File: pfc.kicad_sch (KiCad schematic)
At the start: 58 parts, among them Q3 IRF740, U1 LM324, U2 LMV7219M5, U3 TC4427, U5 74HC00, U6 74LVC1G08

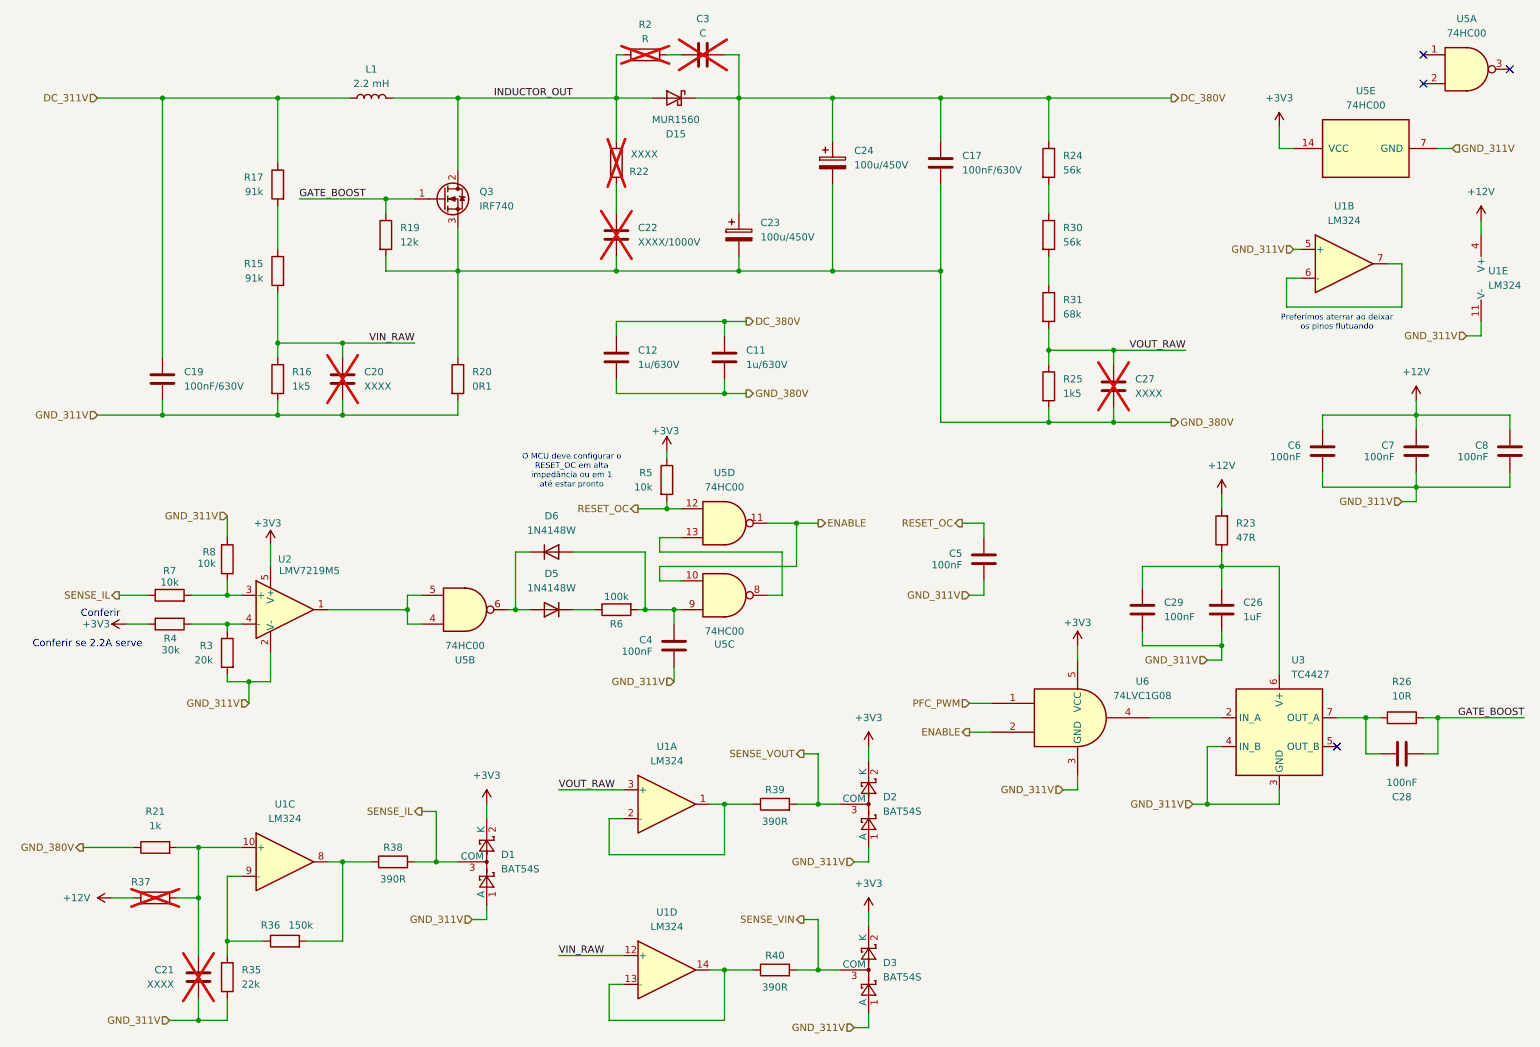
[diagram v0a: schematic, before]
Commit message: pcb: atualizar layout 2D da placa e esquematicos
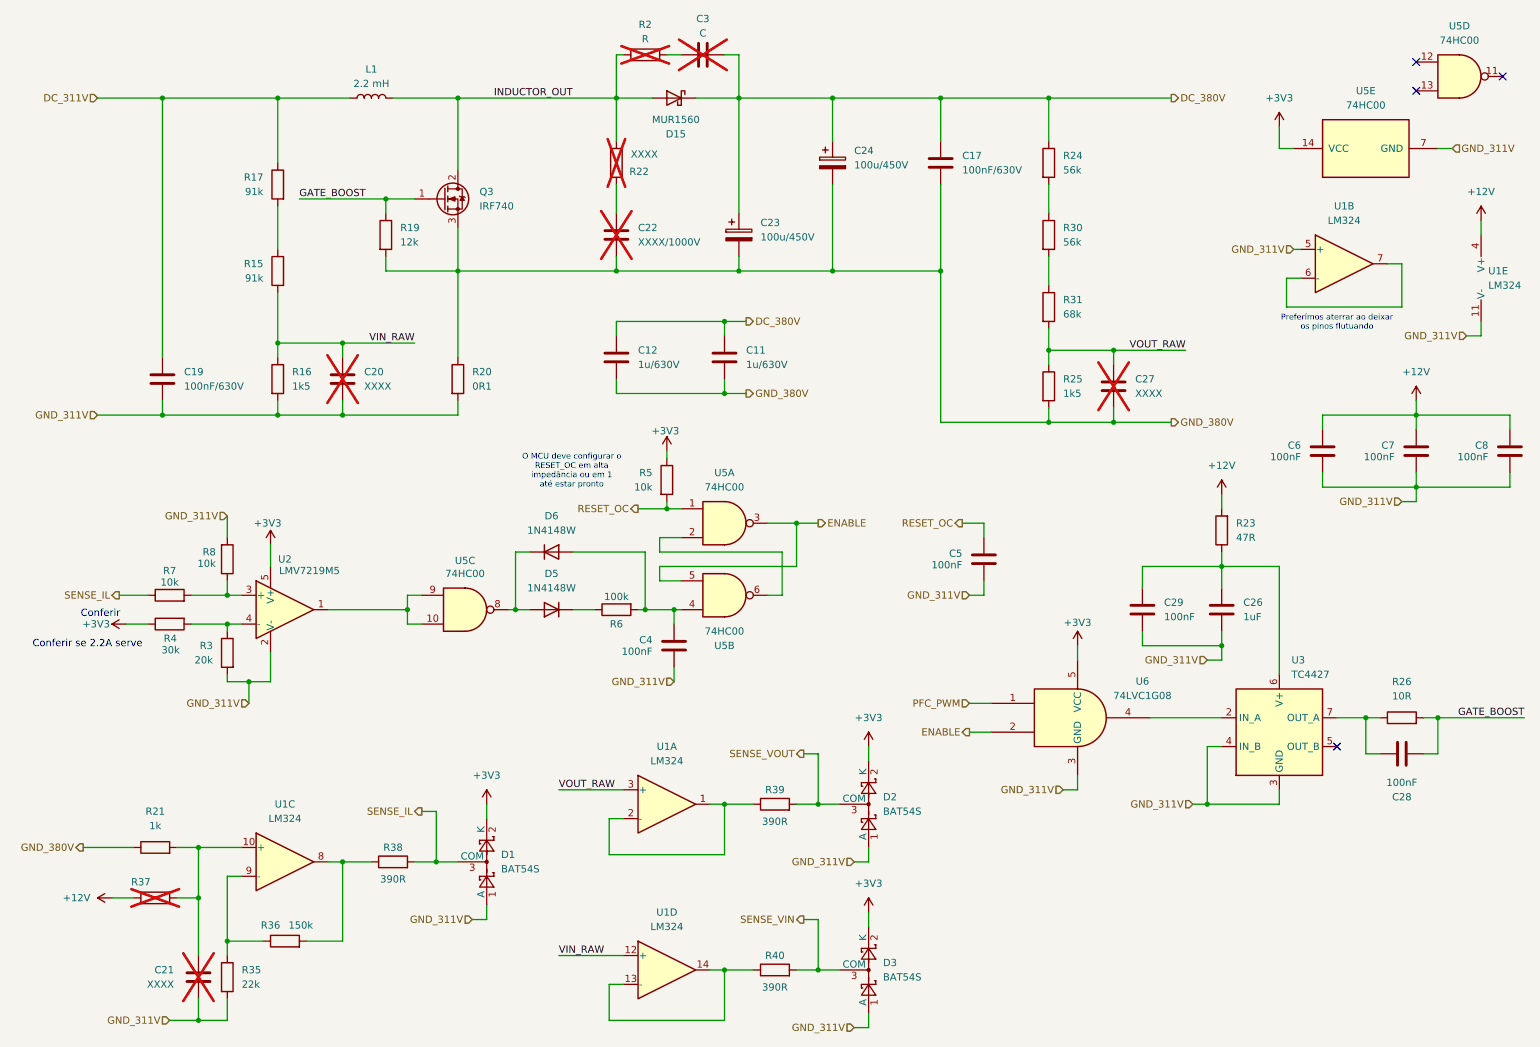
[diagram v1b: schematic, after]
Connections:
- net ENABLE: now also U5.3, U5.5; no longer U5.10, U5.11
- net RESET_OC: now also U5.1; no longer U5.12
- net at U5.8: now also D5.2 (A), D6.1 (K); no longer U5.13
- net at C4.1, D6.2 (A), R6.2: now also U5.4; no longer U5.9
- net at U5.2: now also U5.6
- new net: U2.1, U5.10, U5.9
